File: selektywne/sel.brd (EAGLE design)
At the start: 119.4 x 103.8 mm, 126 parts, among them IC1 TPS70925DBVT, IC2 SP3485EN-L_TR, J1 5-1634556-0, J2 5-1634556-0, J3 5-1634556-0, J4 5-1634556-0, J6 5-1634556-0, J7 5-1634556-0, J8 5-1634556-0, U1 ADS1248IPW, U3 TLC274CN, U4 TPS72301DBVT, U6 TLC274CN, U7 TLC274CN, X2 0446200002

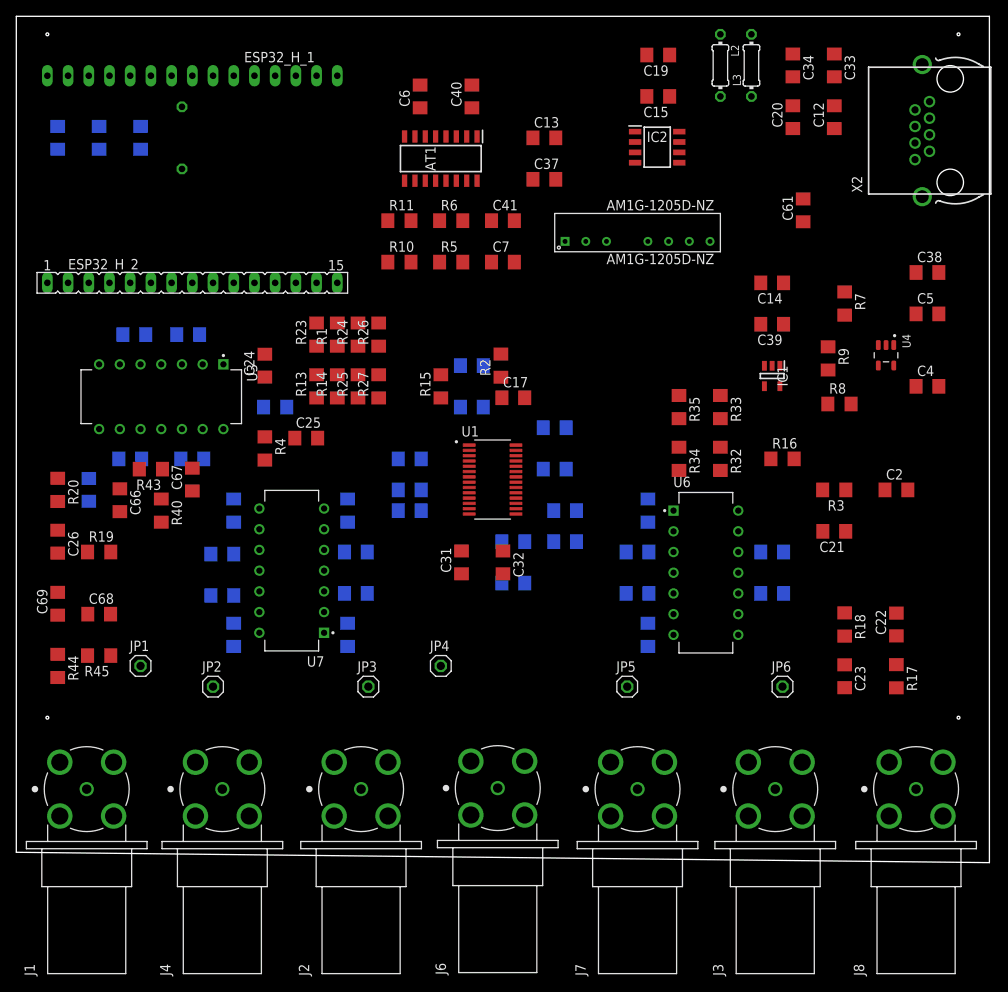
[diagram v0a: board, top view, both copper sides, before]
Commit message: fux wt problem
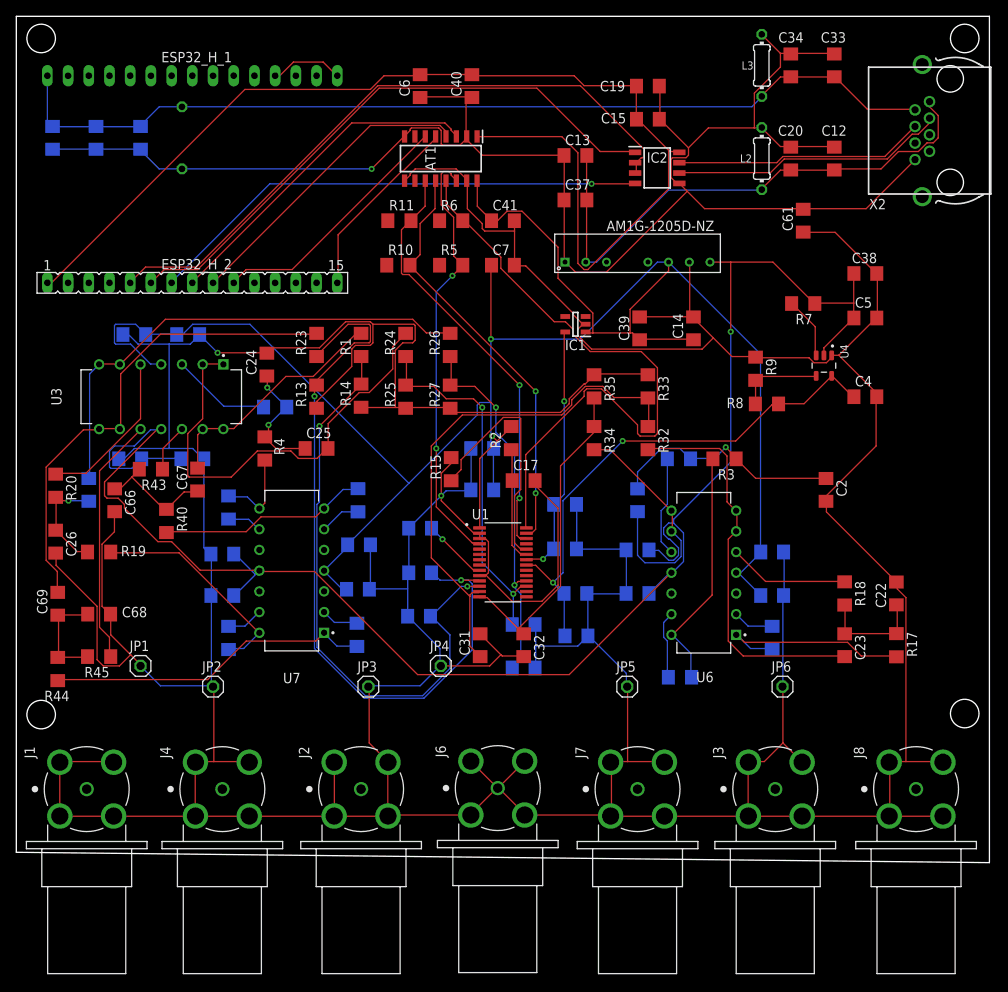
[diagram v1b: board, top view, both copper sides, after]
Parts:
- moved IC1 25.0 mm to (68.6, 64.8), turned to 180 degrees
- moved C21 24.4 mm to (76.2, 43.2), flipped to the bottom, turned to 270 degrees
- moved R42 21.8 mm to (92.7, 26.3), turned to 270 degrees
- moved C52 17.4 mm to (92.7, 31.5), turned to 0 degrees
- moved C56 17.4 mm to (76.2, 37.1), turned to 180 degrees
- moved C51 17.3 mm to (92.7, 36.8), turned to 0 degrees
- moved C55 17.3 mm to (76.2, 31.8), turned to 180 degrees
- moved C39 16.3 mm to (76.5, 64.3), turned to 90 degrees
- moved R3 14.0 mm to (86.9, 48.3)
- moved C1 13.0 mm to (49.4, 29.0)
- moved R16 12.7 mm to (81.3, 48.3), flipped to the bottom, turned to 180 degrees
- moved L2 12.5 mm to (91.4, 85.1)
- moved C9 11.6 mm to (68.7, 26.5)
- moved C14 11.2 mm to (83.1, 64.3), turned to 90 degrees
- moved R34 10.7 mm to (70.9, 50.8)
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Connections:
- net 1IN+_2 renamed WT5
- removed net 2IN+_2: U6.5
- removed net 4IN+_2: R16.1, U6.12
- removed net N$27: R41.1, U6.6
- new net 3IN+_2: R16.1, U6.10
- new net N$1: R41.1, U6.13
- new net WT6: U6.12
- net N$3: now also U6.5; no longer U6.10
- net OUT5: now also U6.6, U6.7; no longer U6.8, U6.9
- net OUT6: now also U6.8, U6.9; no longer U6.13, U6.14
- net OUT6_WT: now also U6.14; no longer U6.7
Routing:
- net GND_OP: track 0.00 -> 795.3 mm, vias 0 -> 2
- net 5V_OP: track 0.00 -> 257.8 mm, vias 0 -> 2
- net -5V_OP: track 0.00 -> 210.3 mm, vias 0 -> 1
- net GND: track 0.00 -> 203.8 mm, vias 0 -> 1
- net +3V3: track 0.00 -> 141.7 mm
- net +5V: track 0.00 -> 116.7 mm
- net CH0: track 0.00 -> 92.2 mm, vias 0 -> 2
- net DIR: track 0.00 -> 79.9 mm
- net CLK_SPI: track 0.00 -> 78.4 mm
- net CH1: track 0.00 -> 73.1 mm, vias 0 -> 2
- net RX2: track 0.00 -> 72.6 mm
- net +12V: track 0.00 -> 67.7 mm
- net -2_5V_OP: track 0.00 -> 65.1 mm, vias 0 -> 2
- net CH4: track 0.00 -> 64.0 mm
- net TX2: track 0.00 -> 62.0 mm, vias 0 -> 1
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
